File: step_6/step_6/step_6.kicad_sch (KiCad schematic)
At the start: 17 parts, among them J2 Conn_01x05_Pin, J3 Conn_01x05_Pin, Q1 BC547, Q2 BC547, SW1 SW_SPDT, U2 SN74HC08N

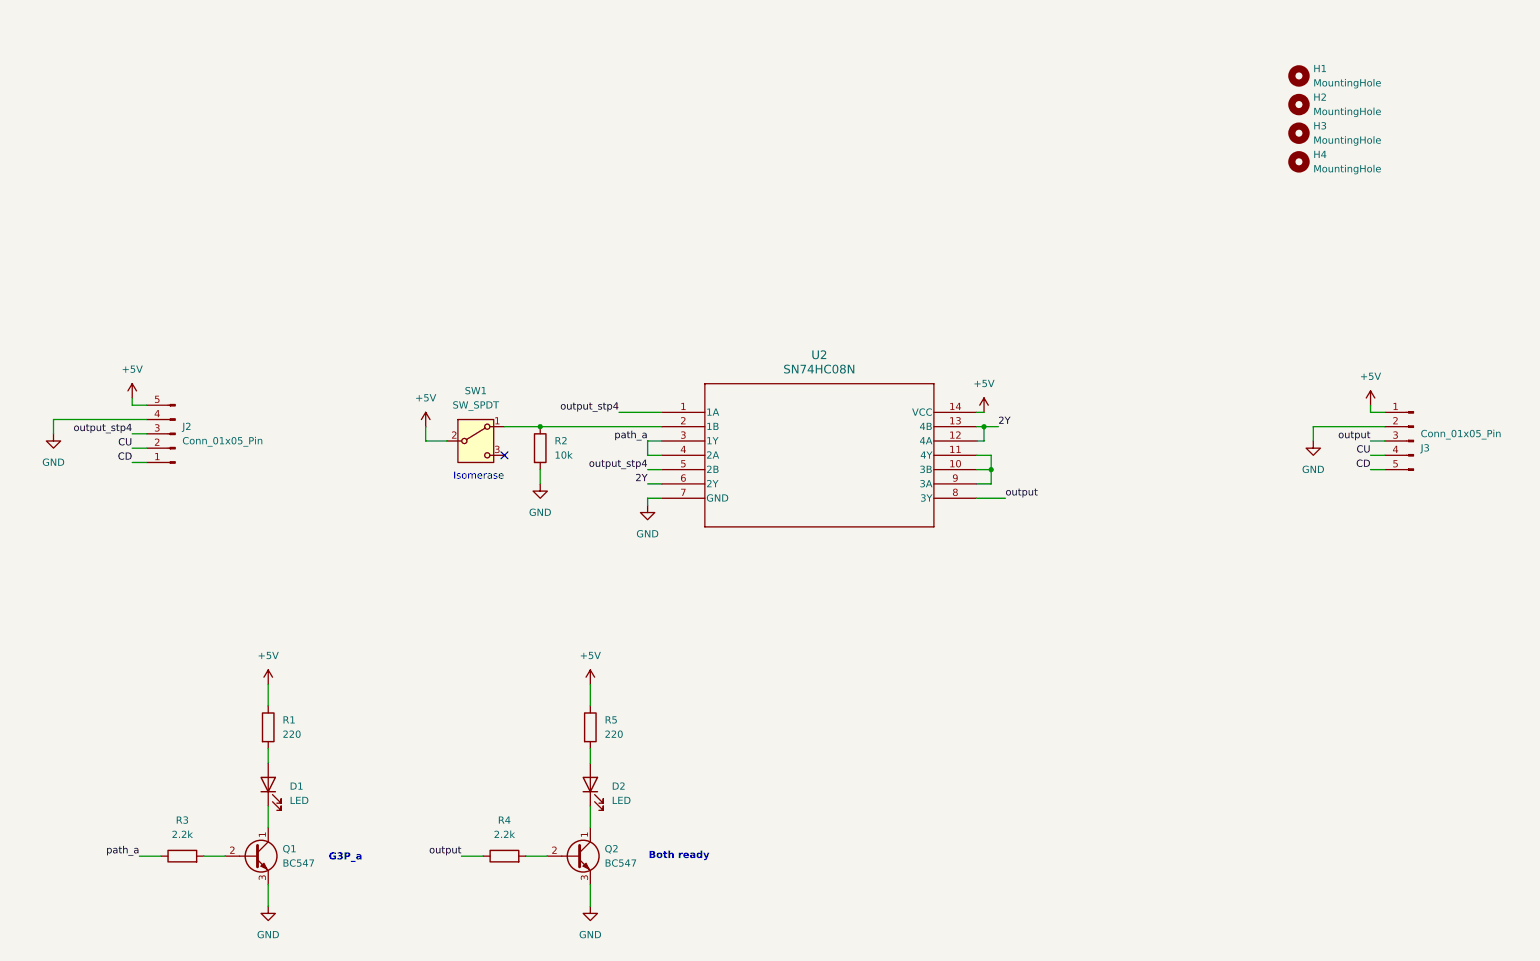
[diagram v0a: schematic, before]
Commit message: all
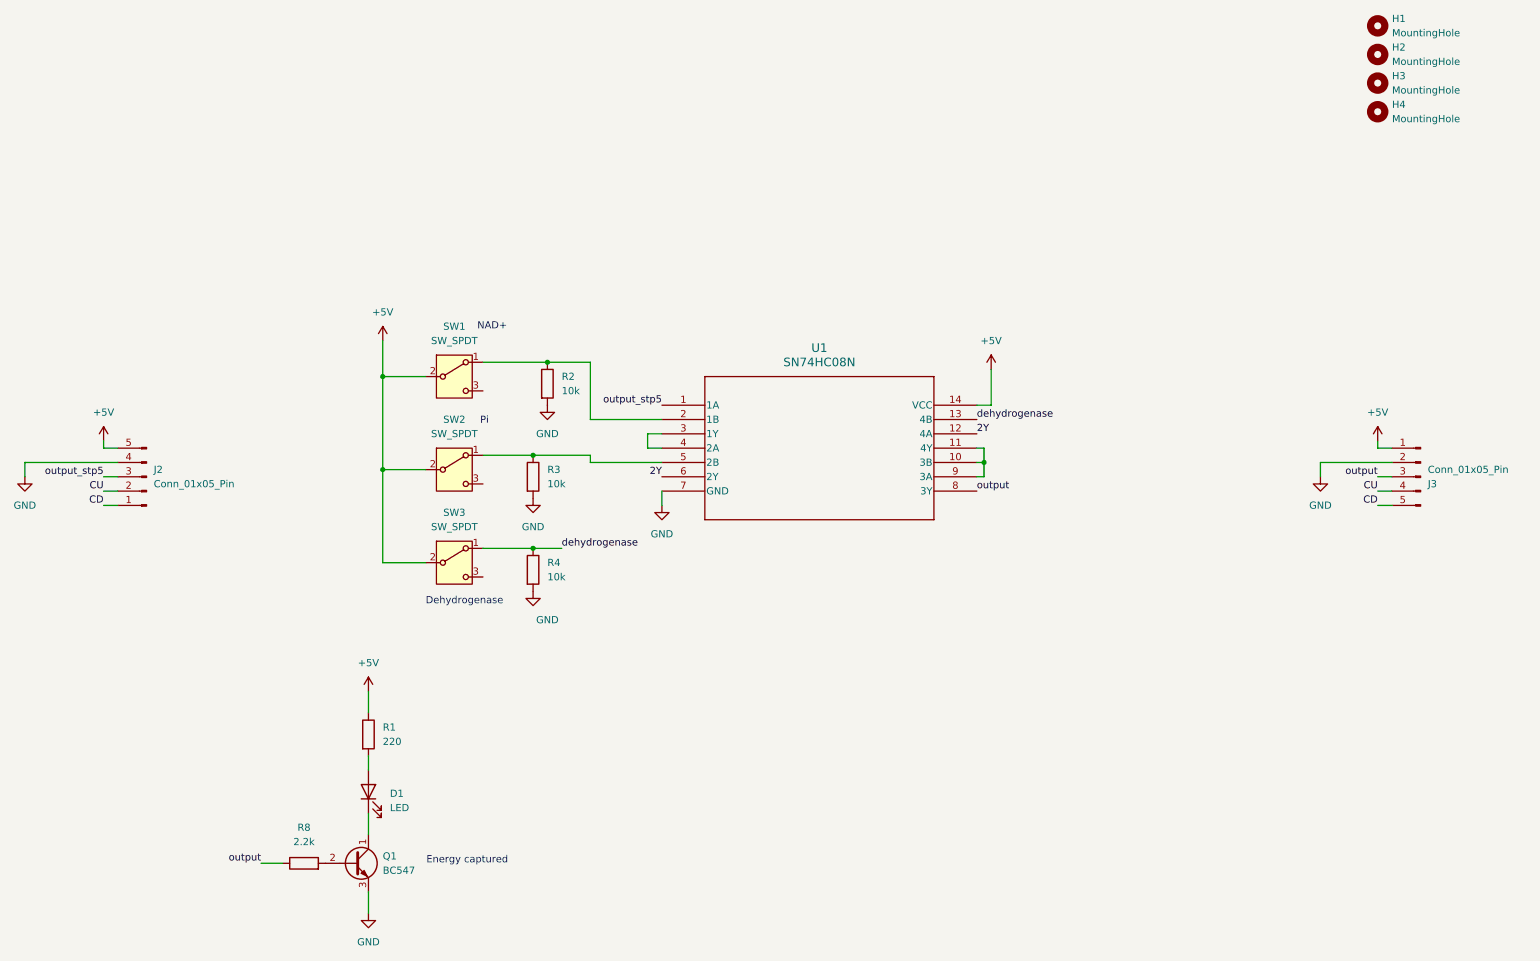
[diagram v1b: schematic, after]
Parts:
- removed D2: LED, LED_THT:LED_D5.0mm, symbol Device:LED
- removed Q2: BC547, Package_TO_SOT_THT:TO-92_Inline, symbol Transistor_BJT:BC547
- removed R5: 220, Resistor_THT:R_Axial_DIN0207_L6.3mm_D2.5mm_P10.16mm_Horizontal, symbol Device:R
- removed U2: SN74HC08N, Package_DIP:DIP-14_W7.62mm_LongPads, symbol SN74HC08N:SN74HC08N
- added R8: 2.2k, Resistor_THT:R_Axial_DIN0207_L6.3mm_D2.5mm_P10.16mm_Horizontal, symbol Device:R
- added SW2, SW3: SW_SPDT, Button_Switch_THT:SW_Slide-03_Wuerth-WS-SLTV_10x2.5x6.4_P2.54mm, symbol Switch:SW_SPDT
- added U1: SN74HC08N, Package_DIP:DIP-14_W7.62mm_LongPads, symbol SN74HC08N:SN74HC08N
- R3, R4: value 2.2k -> 10k; mouser 603-CFR-25JT-52-220R -> 603-CFR-25JB-52-10K
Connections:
- net +5V: now also SW2.2 (B), SW3.2 (B), U1.14 (VCC)
- net 2Y: now also U1.12 (4A), U1.6 (2Y)
- net GND: now also R3.2, R4.2, U1.7 (GND)
- net output: now also R8.1, U1.8 (3Y); no longer R4.1
- net at Q1.2 (B): now also R8.2; no longer R3.2
- net at R2.1, SW1.1 (A): now also U1.2 (1B)
- net output_stp4 renamed output_stp5
- net output_stp5: now also U1.1 (1A)
- net path_a: no longer names the net of R3.1
- net path_a: now also SW2.1 (A), U1.5 (2B)
- new net: U1.10 (3B), U1.11 (4Y), U1.9 (3A)
- new net: U1.3 (1Y), U1.4 (2A)
- new net dehydrogenase: R4.1, SW3.1 (A), U1.13 (4B)
- no-connect marks 1 -> 0
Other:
- note added: "Dehydrogenase"
- note added: "Energy captured"
- note added: "NAD+"
- note added: "Pi"
- note removed: "Both ready"
- note removed: "G3P_a"
- note removed: "Isomerase"
